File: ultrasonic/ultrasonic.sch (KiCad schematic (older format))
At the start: 14 parts, among them J1 Conn_01x23_Female, J2 Conn_01x23_Female, J3 Conn_01x07_Female, J4 HY2.0-2Y, J5 Conn_01x04_Male, Q1 S8050, Q2 S8050, Q3 S8050, Q4 S8050, U1 HAL2481L

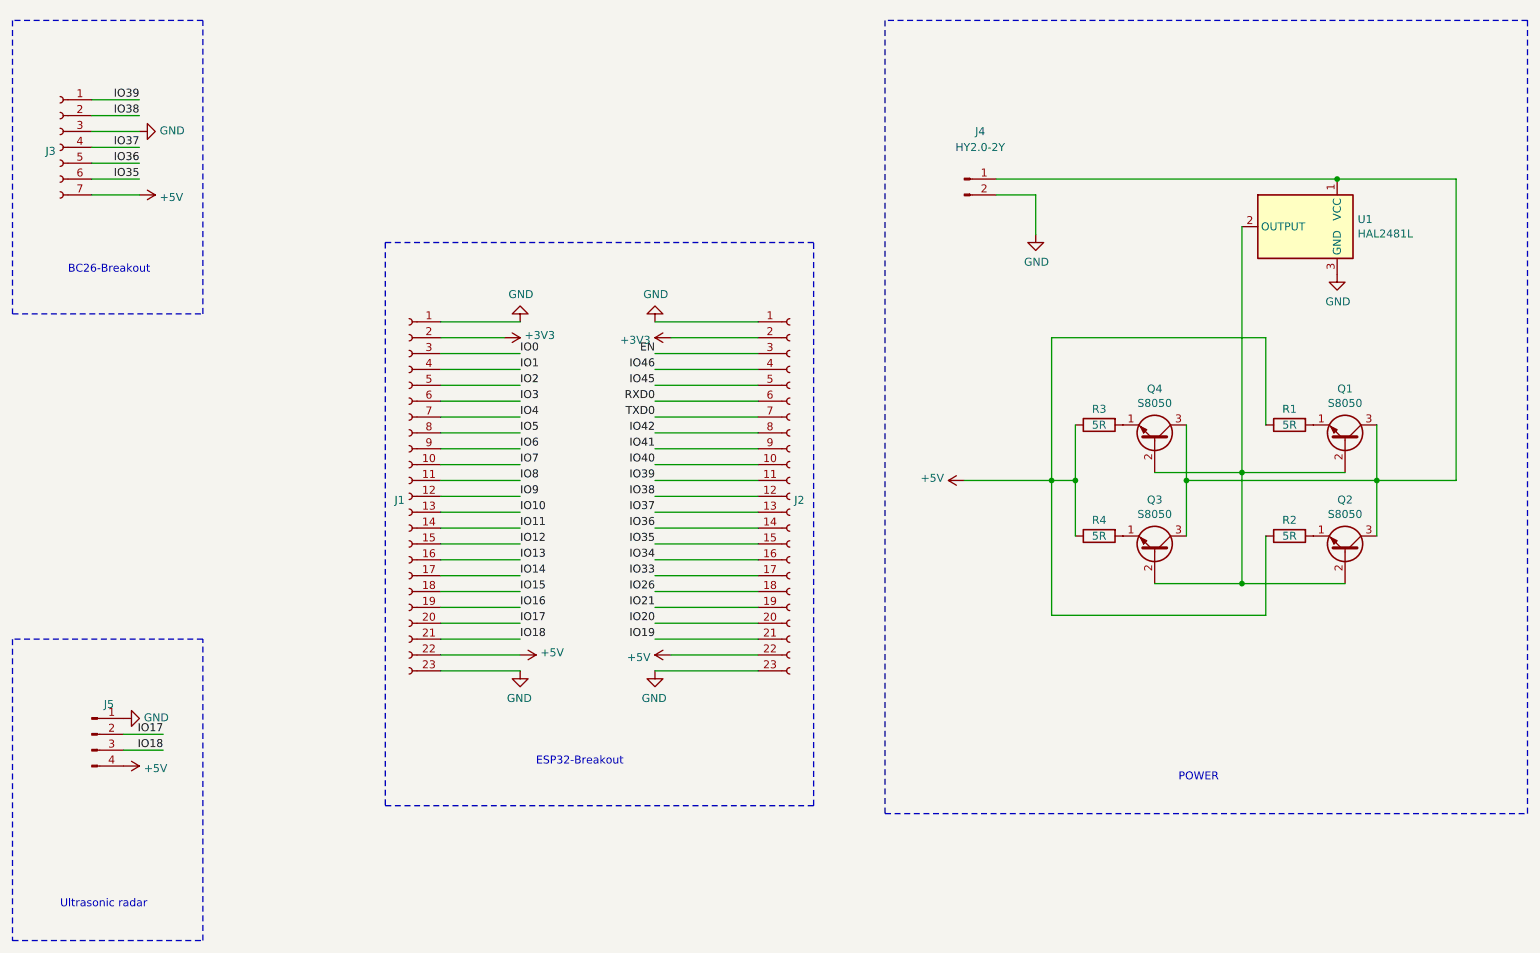
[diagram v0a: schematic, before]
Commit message: feat(network): add network
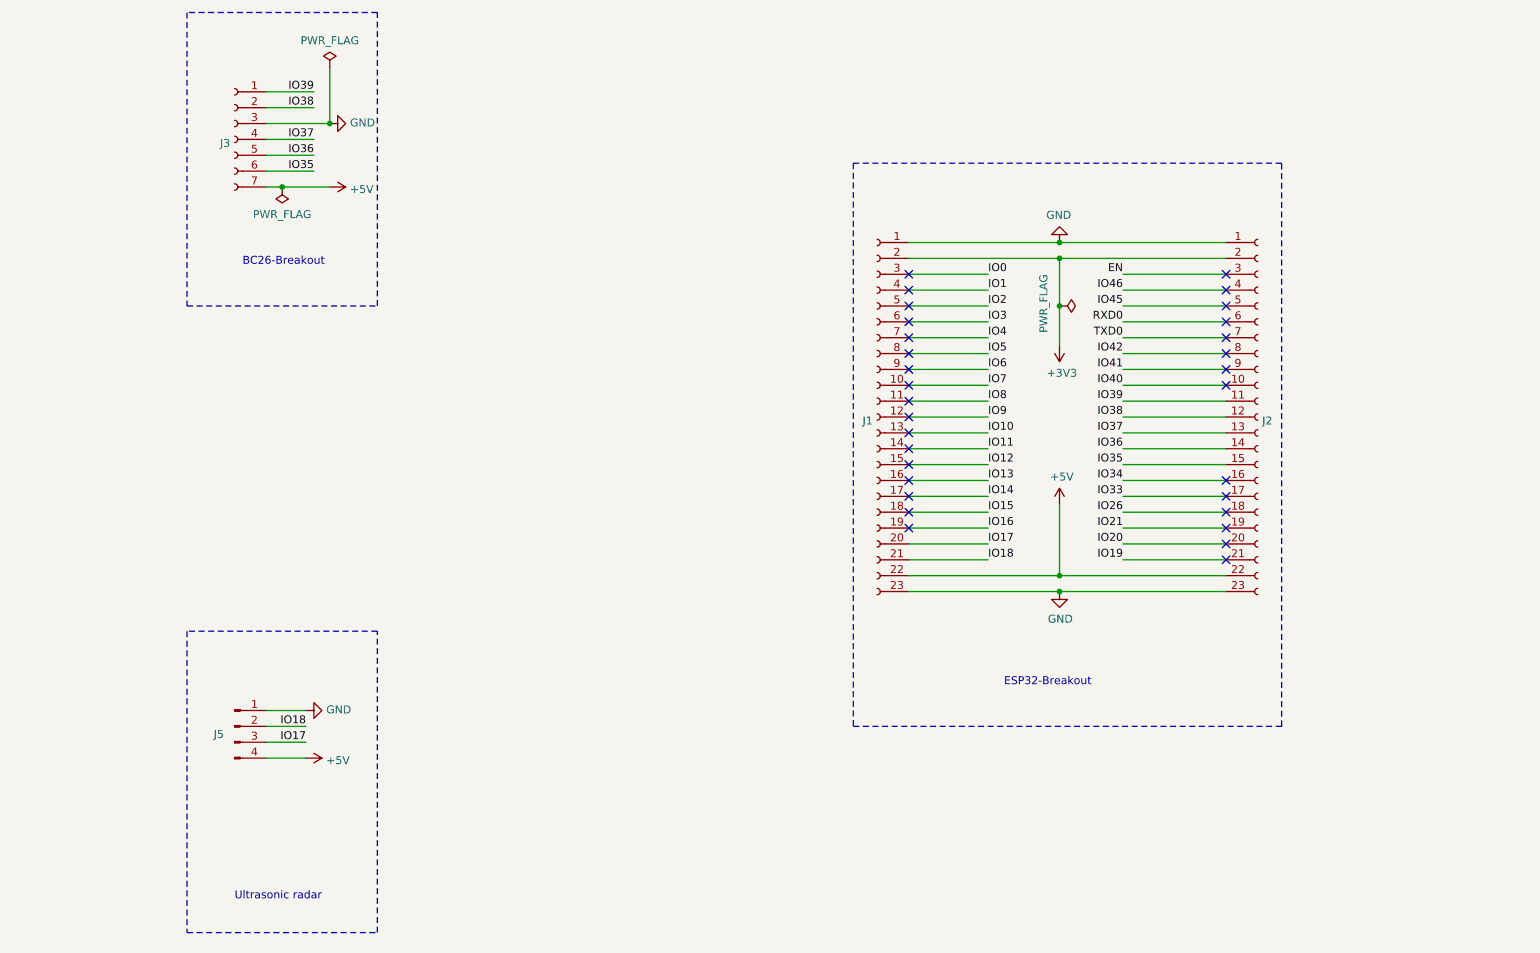
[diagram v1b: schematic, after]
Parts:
- removed J4: HY2.0-2Y, Connector_JST:JST_PH_B2B-PH-K_1x02_P2.00mm_Vertical, symbol Connector:Conn_01x02_Male
- removed Q1, Q2, Q3, Q4: S8050, Package_TO_SOT_THT:TO-92_Inline, symbol Transistor_BJT:S8050
- removed R1, R2, R3, R4: 5R, Capacitor_SMD:C_0603_1608Metric, symbol Device:R
- removed U1: HAL2481L, Package_TO_SOT_SMD:SOT-23, symbol Sensor_Magnetic:SM353LT
- J1: footprint Connector_PinHeader_2.54mm:PinHeader_1x23_P2.54mm_Vertical -> Connector_PinSocket_2.54mm:PinSocket_1x23_P2.54mm_Vertical_SMD_Pin1Right
- J2: footprint Connector_PinHeader_2.54mm:PinHeader_1x23_P2.54mm_Vertical -> Connector_PinHeader_2.54mm:PinHeader_1x23_P2.54mm_Vertical_SMD_Pin1Left
- J3: footprint Connector_PinHeader_2.54mm:PinHeader_1x07_P2.54mm_Vertical -> Connector_JST:JST_PH_S7B-PH-SM4-TB_1x07-1MP_P2.00mm_Horizontal
- J5: footprint (none) -> Connector_JST:JST_PH_S4B-PH-SM4-TB_1x04-1MP_P2.00mm_Horizontal
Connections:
- net IO17: now also J5.3 (Pin_3); no longer J5.2 (Pin_2)
- net IO18: now also J5.2 (Pin_2); no longer J5.3 (Pin_3)
- no-connect marks 0 -> 31
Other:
- note removed: "POWER"
- moved on the sheet: J1, J2, J3, J5

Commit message: new release
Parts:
- J2: footprint Connector_PinHeader_2.54mm:PinHeader_1x23_P2.54mm_Vertical_SMD_Pin1Left -> Connector_PinSocket_2.54mm:PinSocket_1x23_P2.54mm_Vertical_SMD_Pin1Left
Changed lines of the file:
@@
 F 0 "J2" H 9378 3626 50  0000 L CNN
 F 1 "Conn_01x23_Female" H 9378 3535 50  0001 L CNN
-F 2 "Connector_PinHeader_2.54mm:PinHeader_1x23_P2.54mm_Vertical_SMD_Pin1Left" H 9350 3650 50  0001 C CNN
+F 2 "Connector_PinSocket_2.54mm:PinSocket_1x23_P2.54mm_Vertical_SMD_Pin1Left" H 9350 3650 50  0001 C CNN
 F 3 "~" H 9350 3650 50  0001 C CNN
 	1    9350 3650

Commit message: change pinhead to left
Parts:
- J1: footprint Connector_PinSocket_2.54mm:PinSocket_1x23_P2.54mm_Vertical_SMD_Pin1Right -> Connector_PinSocket_2.54mm:PinSocket_1x23_P2.54mm_Vertical_SMD_Pin1Left
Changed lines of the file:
@@
 F 0 "J1" H 6978 3626 50  0000 L CNN
 F 1 "Conn_01x23_Female" H 6978 3535 50  0001 L CNN
-F 2 "Connector_PinSocket_2.54mm:PinSocket_1x23_P2.54mm_Vertical_SMD_Pin1Right" H 6950 3650 50  0001 C CNN
+F 2 "Connector_PinSocket_2.54mm:PinSocket_1x23_P2.54mm_Vertical_SMD_Pin1Left" H 6950 3650 50  0001 C CNN
 F 3 "~" H 6950 3650 50  0001 C CNN
 	1    6950 3650
